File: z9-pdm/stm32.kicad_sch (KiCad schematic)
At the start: 56 parts, among them J4 Conn_ST_STDC14, J5 DF40HC3.0-100DS-0.4V51, J7 Conn_TagConnect_2070, SW1 Tactile Button, 160gf, SW2 Tactile Button, 160gf, U3 STM32F427V_G-I_Tx, X1 8MHz 20pF

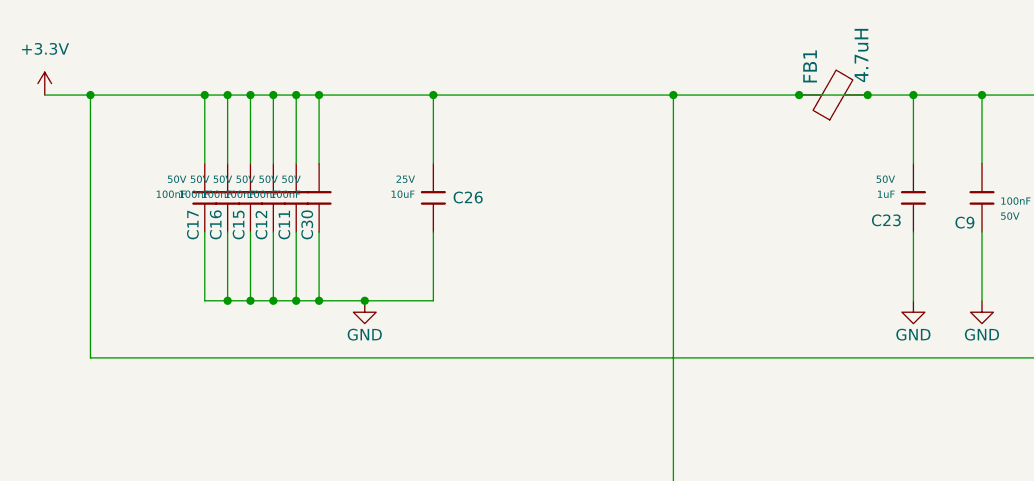
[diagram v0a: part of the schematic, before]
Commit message: x
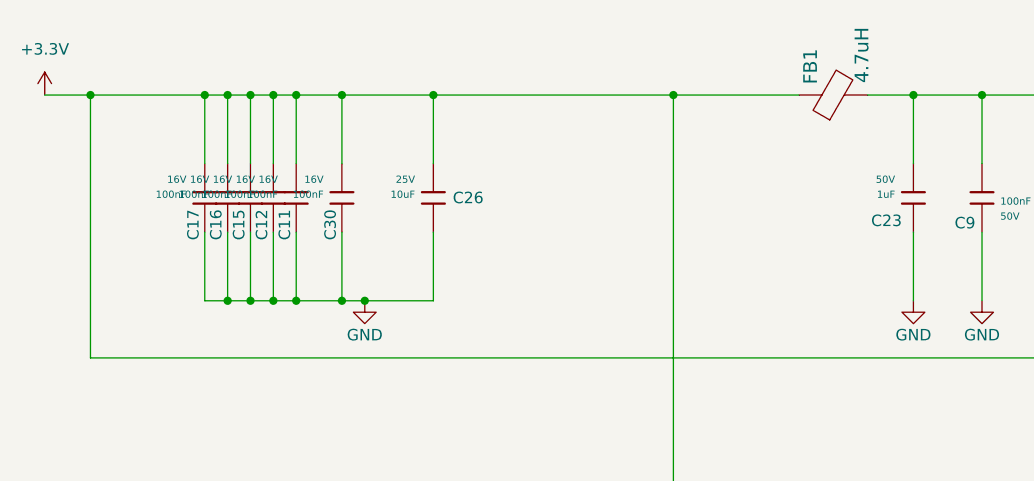
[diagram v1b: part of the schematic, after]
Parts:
- C11, C12, C15, C16, C17, C30: footprint PCM_JLCPCB:C_0603 -> PCM_JLCPCB:C_0402; symbol PCM_JLCPCB-Capacitors:0603,100nF -> dnt_global:0402,100nF, 16V; LCSC C14663 -> C1525; Manufacturer YAGEO -> Samsung Electro-Mechanics; Part CC0603KRX7R9BB104 -> CL05B104KO5NNNC; Price 0.006USD -> 0.004USD; Stock 70324515 -> 20208285; Voltage Rated 50V -> 16V
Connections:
- net +3.3V: no longer C23.2, C9.1, FB1.2, U3.22 (VDDA)
- new net: C23.2, C9.1, FB1.2, U3.22 (VDDA)
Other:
- moved on the sheet: C30
